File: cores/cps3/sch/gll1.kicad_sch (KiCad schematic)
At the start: 1 part, among them J11 DL-3429-GLL1

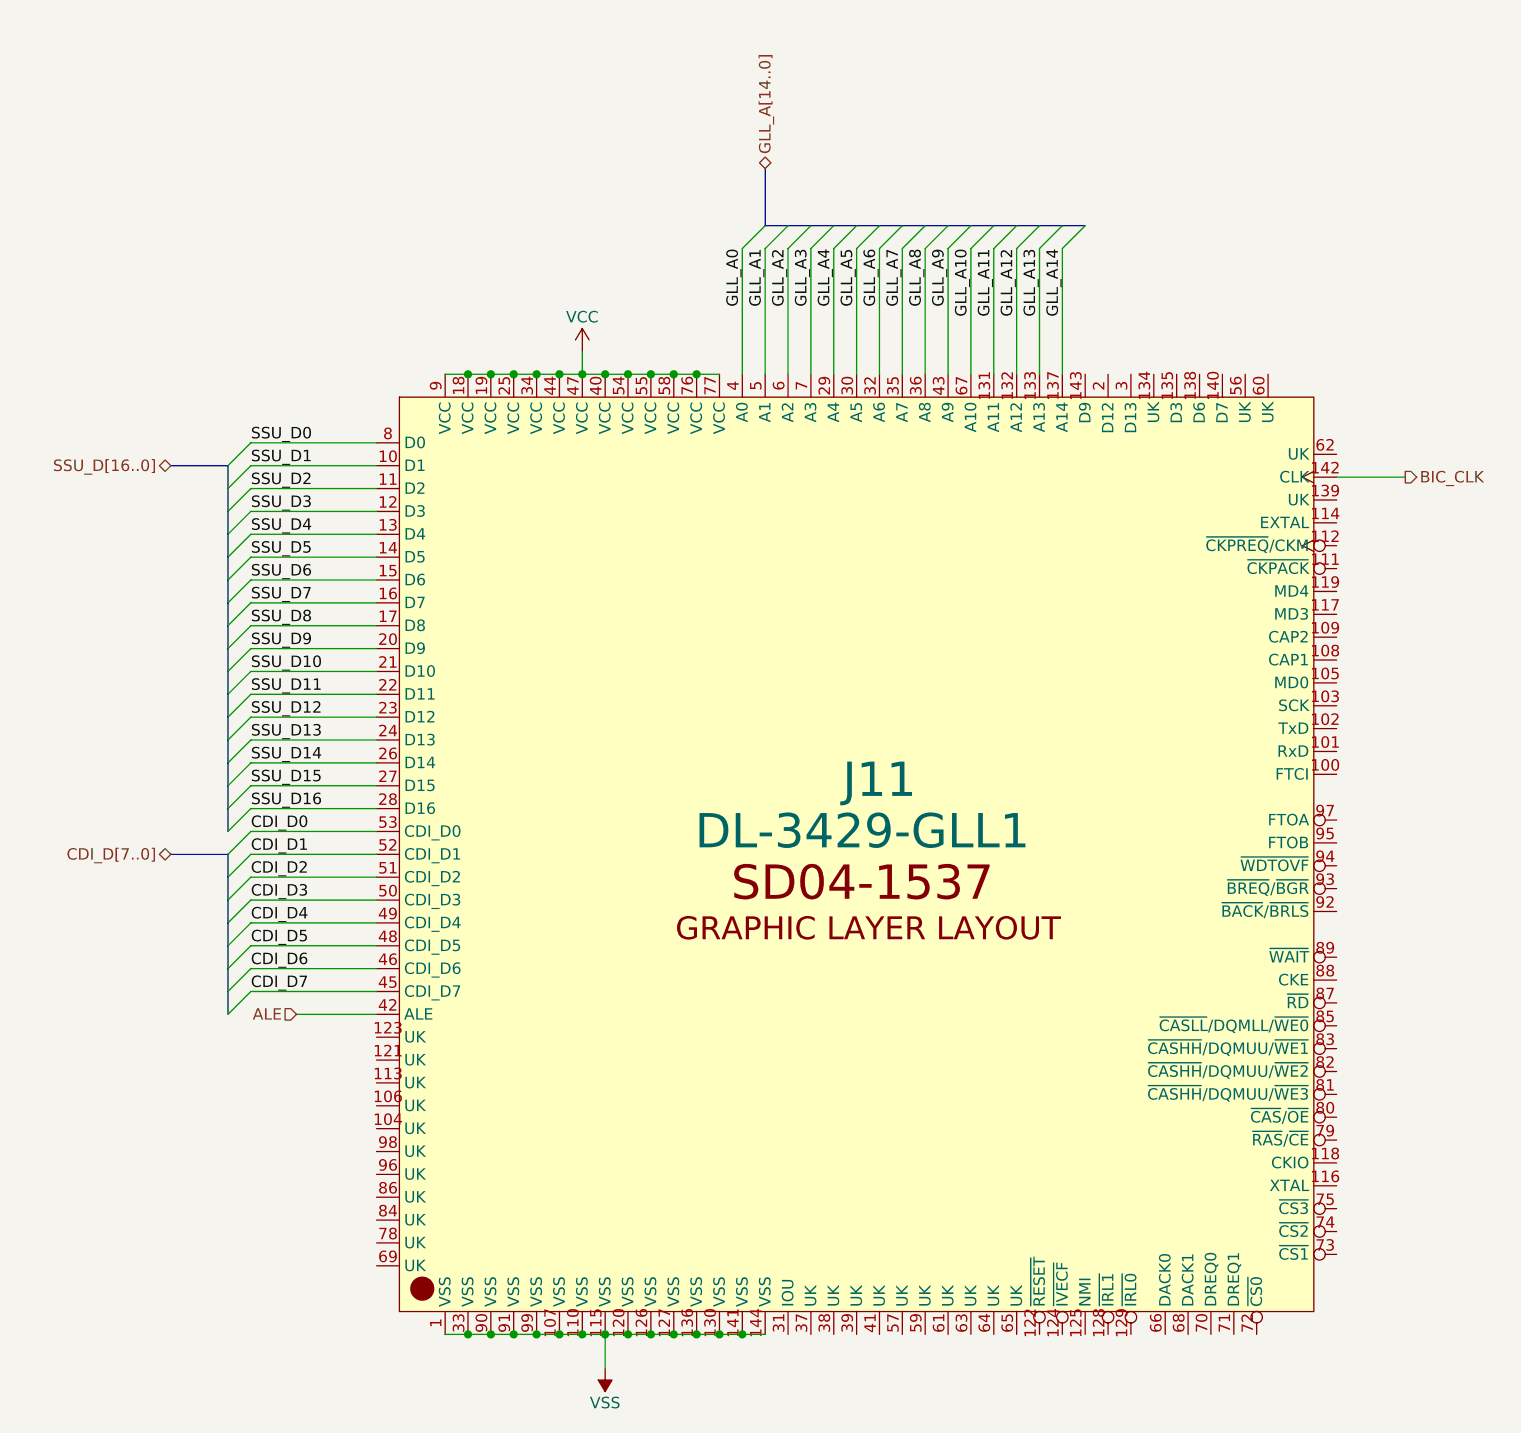
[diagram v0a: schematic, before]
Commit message: iou
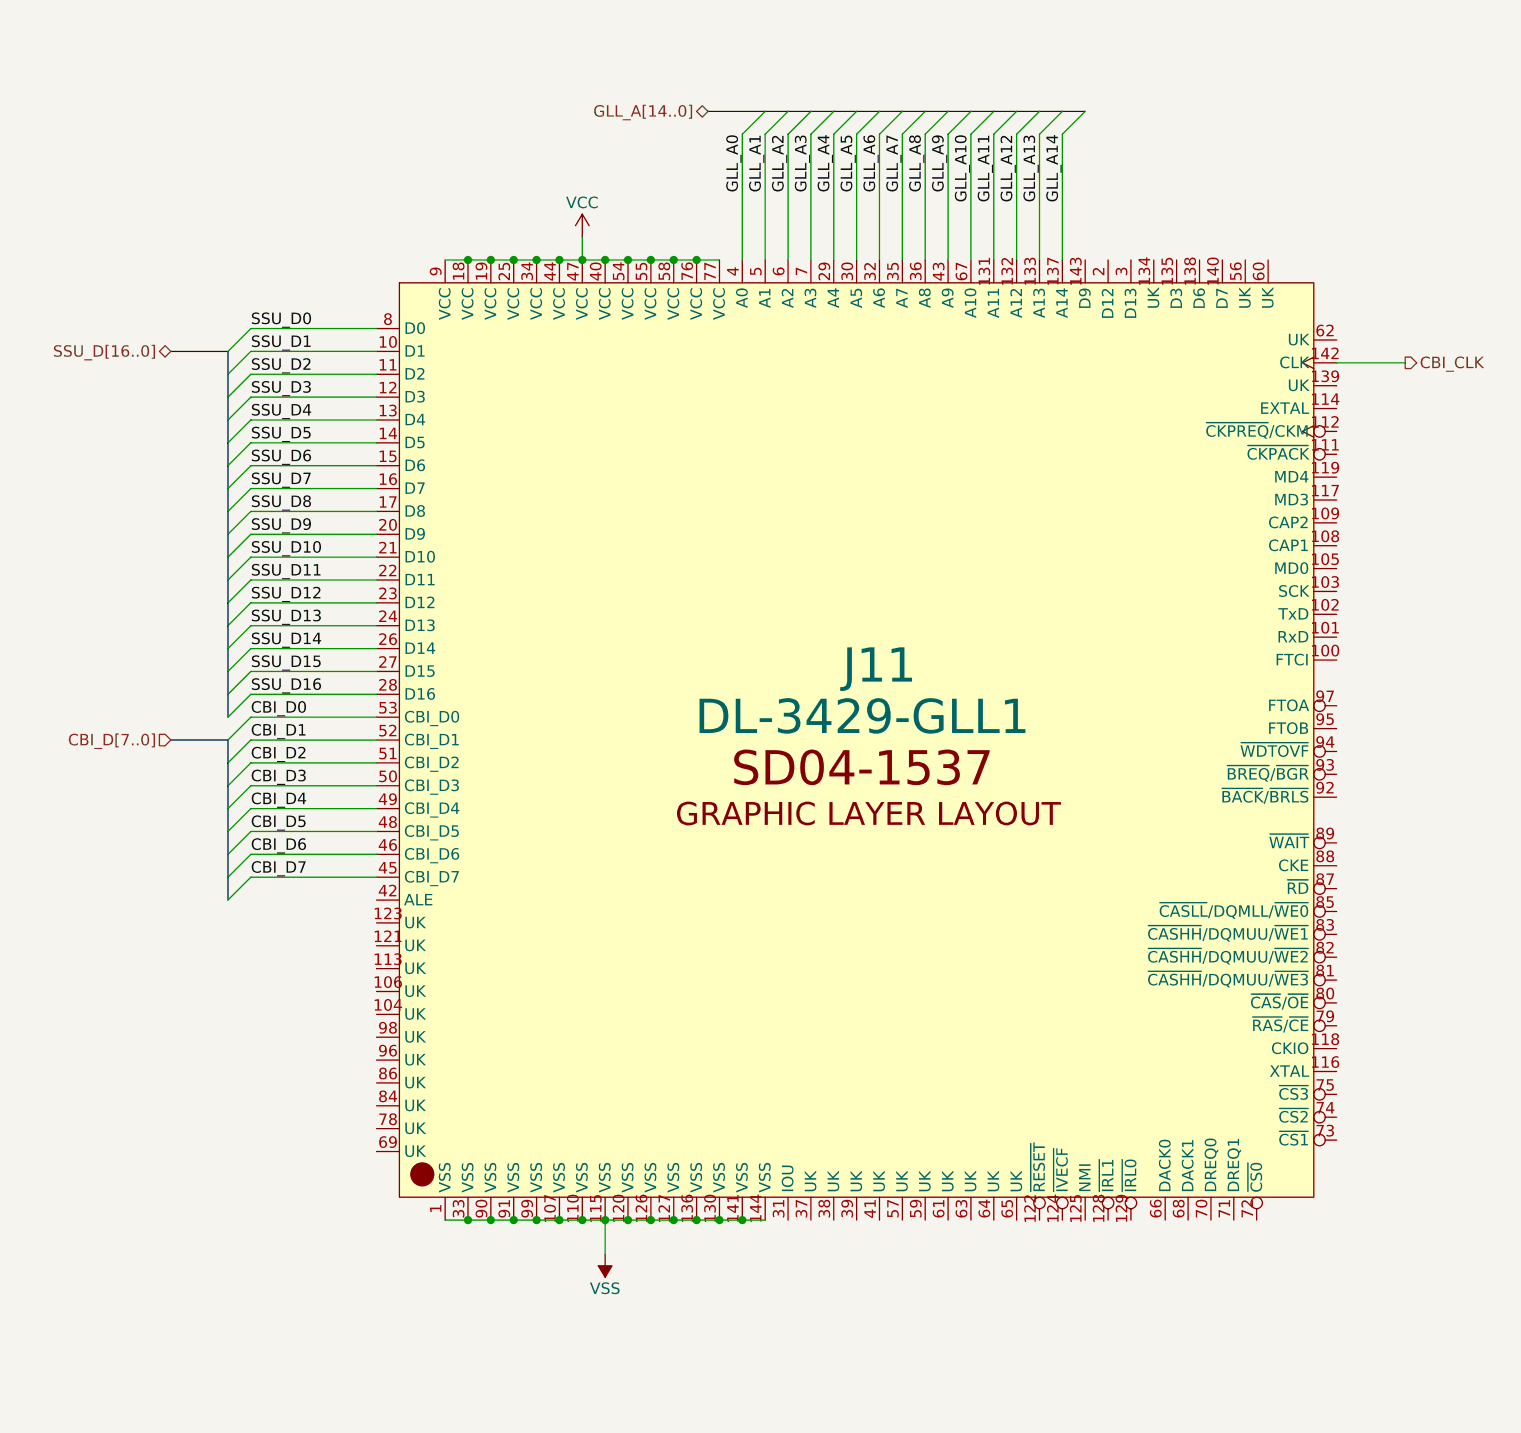
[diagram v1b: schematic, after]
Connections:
- net ALE: no longer names the net of J11.42 (ALE)
- net BIC_CLK renamed CBI_CLK
- net CDI_D0 renamed CBI_D0
- net CDI_D1 renamed CBI_D1
- net CDI_D2 renamed CBI_D2
- net CDI_D3 renamed CBI_D3
- net CDI_D4 renamed CBI_D4
- net CDI_D5 renamed CBI_D5
- net CDI_D6 renamed CBI_D6
- net CDI_D7 renamed CBI_D7
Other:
- moved on the sheet: J11
